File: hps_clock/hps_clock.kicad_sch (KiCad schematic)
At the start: 34 parts, among them J1 Barrel_Jack_Switch, J2 Conn_01x06, SW1 Omron_B3F_SPST, SW2 Omron_B3F_SPST, SW3 Omron_B3F_SPST, SW4 Omron_B3F_SPST, U1 DS1307_DIP-8, U2 L7805, U3 ATmega328-PU, Y1 Crystal_16MHz

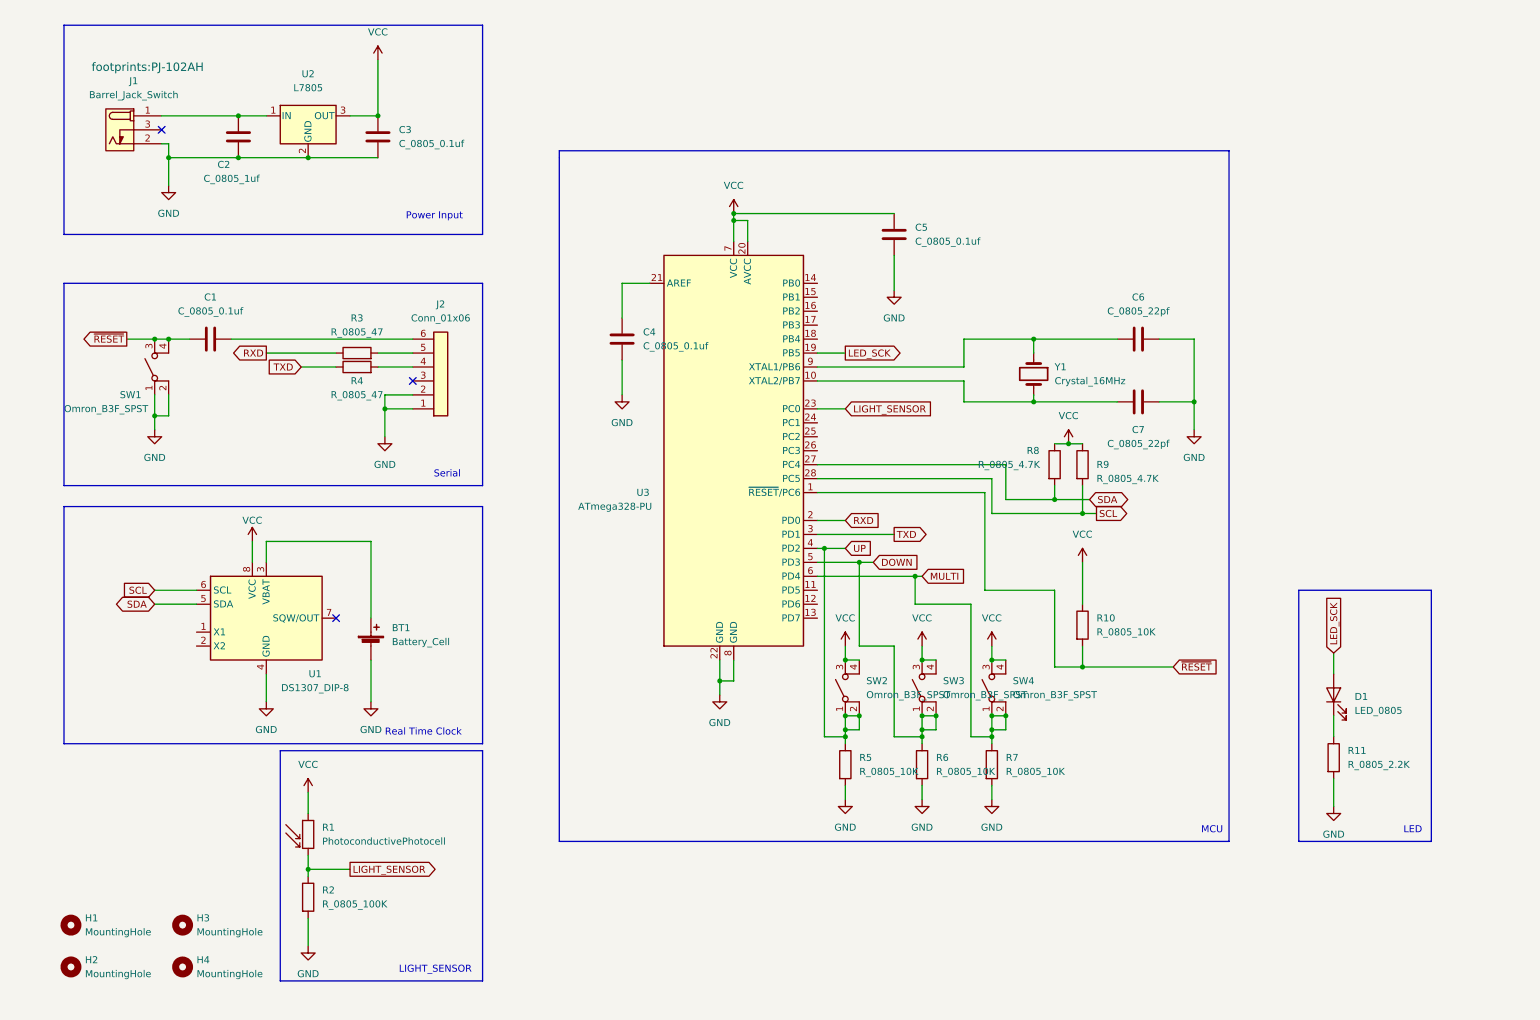
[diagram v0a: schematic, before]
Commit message: schematic done..?
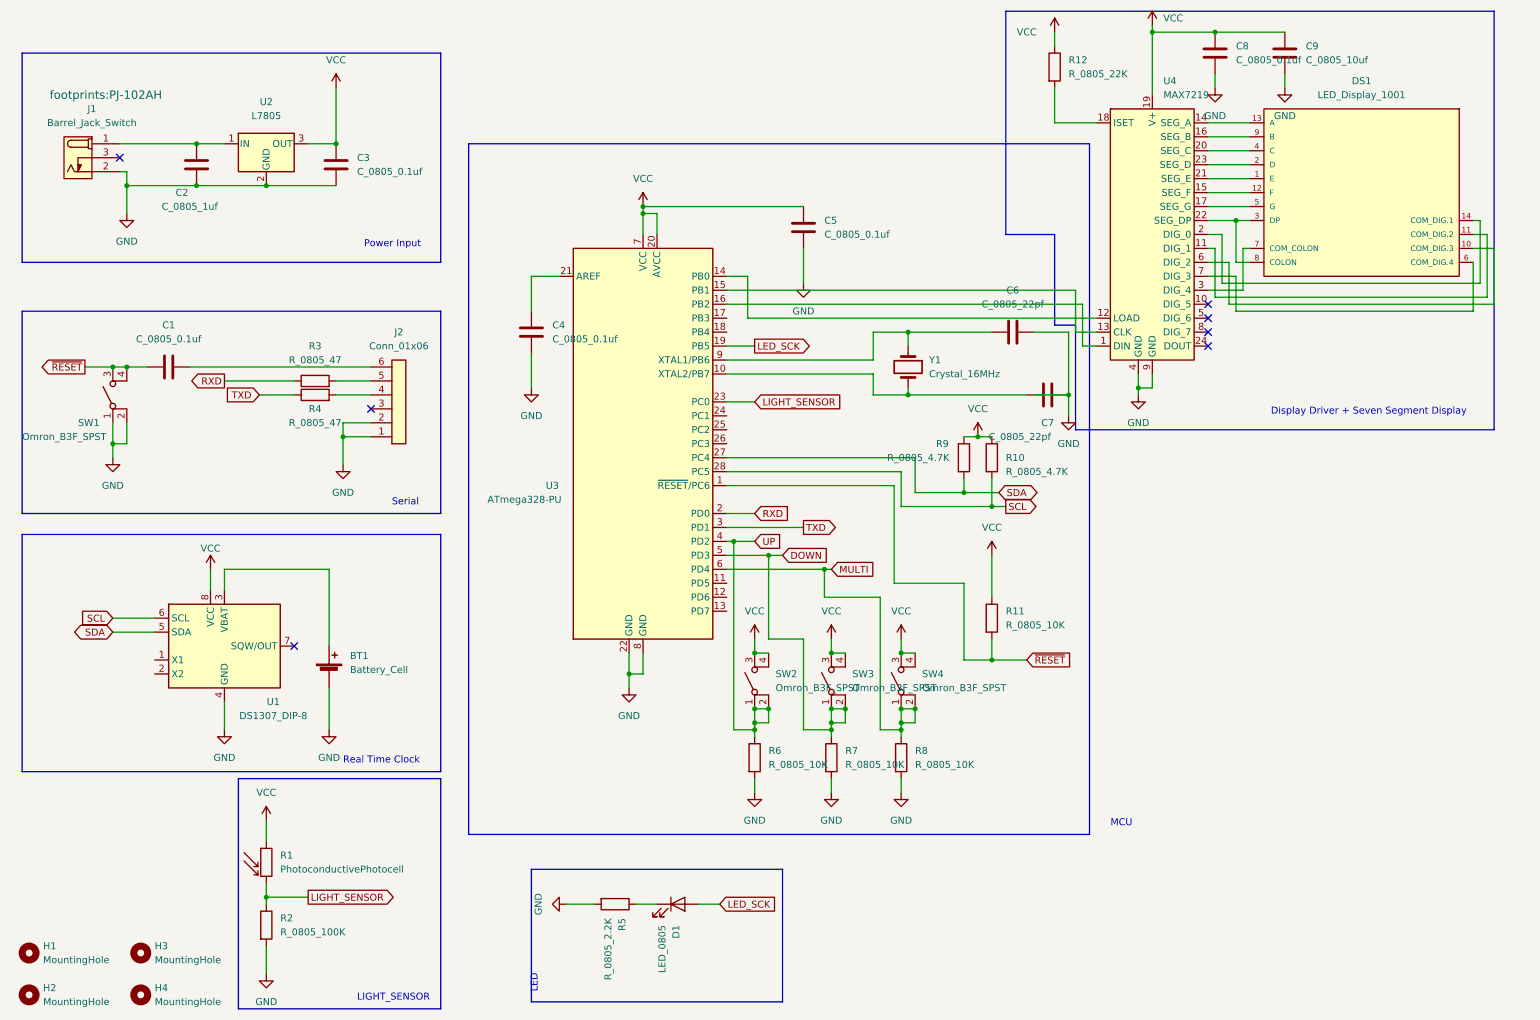
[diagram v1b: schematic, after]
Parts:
- added C8: C_0805_0.1uf, footprints:C_0805_2012Metric, symbol HPS:C_0805_0.1uf
- added C9: C_0805_10uf, footprints:C_0805_2012Metric, symbol HPS:C_0805_10uf
- added DS1: LED_Display_1001, footprints:Adafruit-1001-0-0-MFG, symbol HPS:LED_Display_1001
- added R12: R_0805_22K, footprints:R_0805_2012Metric, symbol HPS:R_0805_22K
- added U4: MAX7219, footprints:DIP-24_W7.62mm, symbol HPS:MAX7219
- U2: footprint (none) -> footprints:TO-252-2
- renumbered R9 to R10, R10 to R11, R11 to R5, R5 to R6, R6 to R7, R7 to R8, R8 to R9
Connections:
- net GND: now also C8.2, C9.2, U4.4 (GND), U4.9 (GND)
- net VCC: now also C8.1, C9.1, R12.1, U4.19 (V+)
- net at U3.14 (PB0): now also U4.12 (LOAD)
- net at U3.15 (PB1): now also U4.13 (CLK)
- net at U3.16 (PB2): now also U4.1 (DIN)
- new net: DS1.1 (E), U4.21 (SEG_E)
- new net: DS1.10 (COM_DIG.3), U4.6 (DIG_2)
- new net: DS1.11 (COM_DIG.2), U4.11 (DIG_1)
- new net: DS1.12 (F), U4.15 (SEG_F)
- new net: DS1.13 (A), U4.14 (SEG_A)
- new net: DS1.14 (COM_DIG.1), U4.2 (DIG_0)
- new net: DS1.2 (D), U4.23 (SEG_D)
- new net: DS1.3 (DP), DS1.8 (COLON), U4.22 (SEG_DP)
- new net: DS1.4 (C), U4.20 (SEG_C)
- new net: DS1.5 (G), U4.17 (SEG_G)
- new net: DS1.6 (COM_DIG.4), U4.7 (DIG_3)
- new net: DS1.7 (COM_COLON), U4.3 (DIG_4)
- new net: DS1.9 (B), U4.16 (SEG_B)
- new net: R12.2, U4.18 (ISET)
- no-connect marks 3 -> 7
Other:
- note added: "Display Driver + Seven Segment Display"
- moved on the sheet: BT1, C1, C2, C3, C4, C5, C6, C7, D1, H1, H2, H3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
